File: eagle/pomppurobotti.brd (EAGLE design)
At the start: 100 x 80 mm, 3 parts

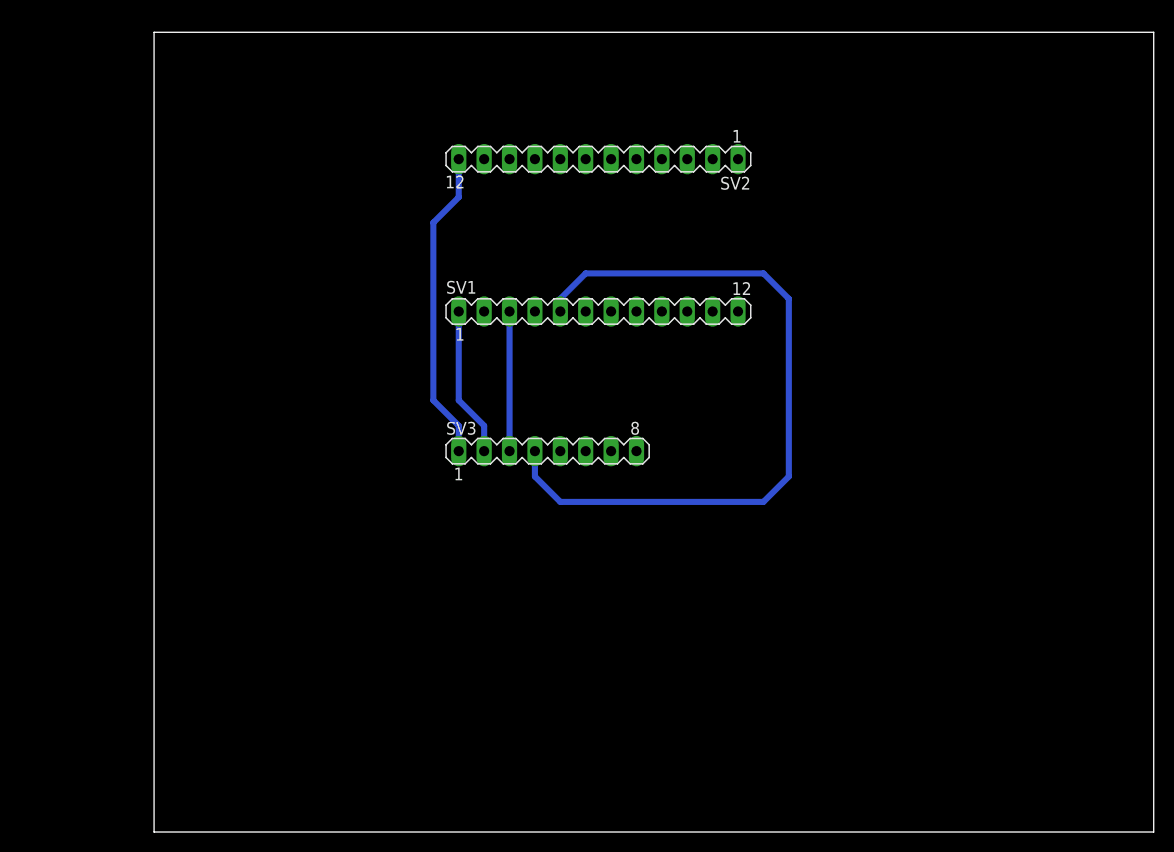
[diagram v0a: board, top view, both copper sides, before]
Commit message: First version of PCB
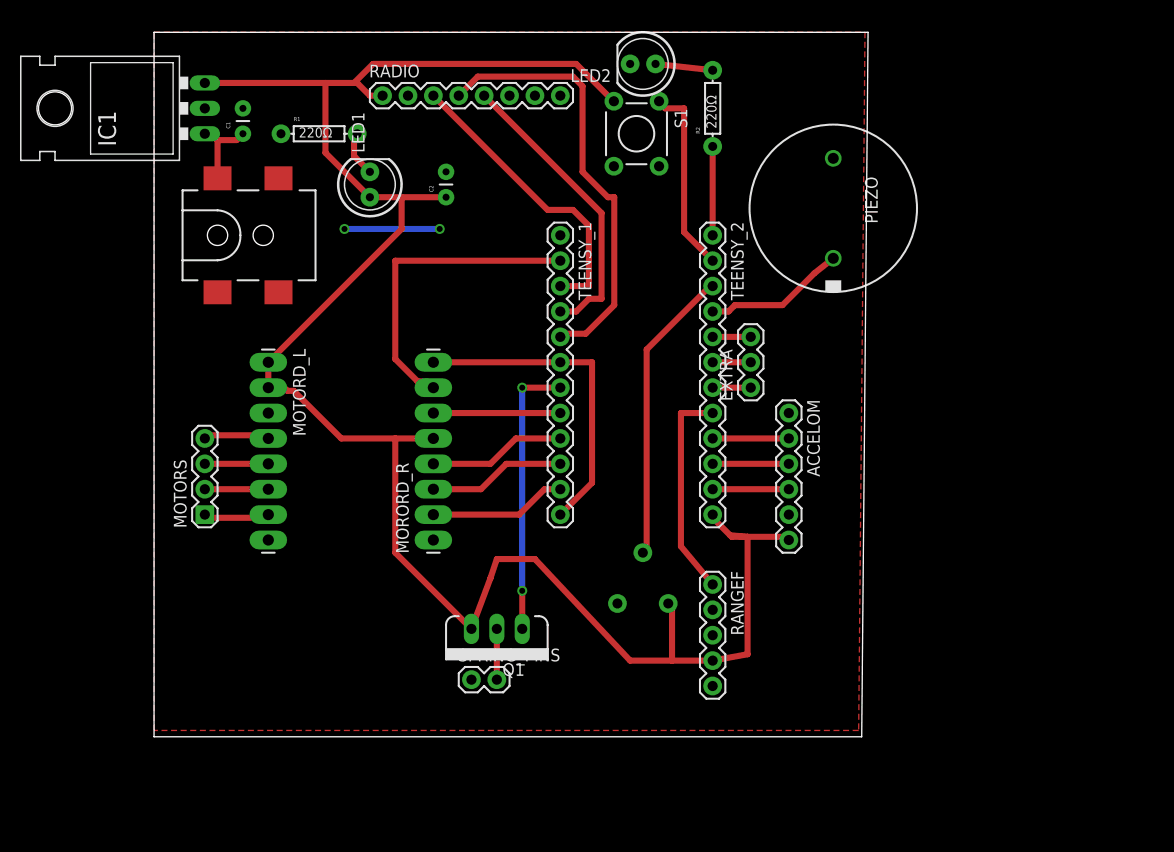
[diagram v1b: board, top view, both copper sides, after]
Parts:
- removed SV1, SV2: (no value), con-lstb:MA12-1
- removed SV3: (no value), con-lstb:MA08-1
- added ACCELOM: (no value), SparkFun-Connectors:1X06
- added C1, C2: 10uF, SparkFun-Capacitors:CAP-PTH-SMALL
- added EXTRA: (no value), SparkFun-Connectors:1X03
- added IC1: (no value), SparkFun-PowerIC:TO-220-ALT
- added JP1: POWER_JACK1, SparkFun-Connectors:POWER_JACK_SMD_OVERPASTE_REDBOARD_0603
- added LED1, LED2: RED, SparkFun-LED:LED5MM
- added MORORD_R, MOTORD_L: (no value), SparkFun-Connectors:1X08_LONGPADS
- added MOTORS: (no value), SparkFun-Connectors:1X04
- added PIEZO: EFBAA40D101, buzzer:EFBAA40D101
- added Q1: MOSFET-NCHANNELFQP30N06L, SparkFun-DiscreteSemi:TO220V
- added R1, R2: 220Ω, SparkFun-Resistors:AXIAL-0.3
- added RADIO: (no value), SparkFun-Connectors:1X08_ROUND
- added RANGEF: (no value), SparkFun-Connectors:1X05
- added RV1: (no value), SparkFun-Electromechanical:TRIM_POT
- added S1: SWITCH-MOMENTARY-2PTH, SparkFun-Electromechanical:TACTILE-PTH
- added SPRING_PINS: M02PTH, SparkFun-Connectors:1X02
- added TEENSY_1, TEENSY_2: M12PTH, SparkFun-Connectors:1X12
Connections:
- removed net +5V: SV2.12, SV3.1
- removed net 0: SV1.2
- removed net 10: SV1.12
- removed net 4: SV1.6
- removed net 5: SV1.7
- removed net 6: SV1.8
- removed net 7: SV1.9
- removed net 8: SV1.10
- removed net 9: SV1.11
- removed net N$14: SV2.11
- removed net N$15: SV2.10
- removed net N$16: SV2.9
- removed net N$17: SV2.8
- removed net N$18: SV2.7
- removed net N$19: SV2.6
- removed net N$20: SV2.5
- removed net N$21: SV2.4
- removed net N$22: SV2.3
- removed net N$23: SV2.2
- removed net N$24: SV2.1
- new net A0: ACCELOM.2, TEENSY_2.9
- new net A01: MOTORD_L.4, MOTORS.4
- new net A02: MOTORD_L.5, MOTORS.3
- new net A1: ACCELOM.3, TEENSY_2.10
- new net A2: ACCELOM.4, TEENSY_2.11
- new net A4: EXTRA.1, TEENSY_2.7
- new net A5: EXTRA.2, TEENSY_2.6
- new net A8: RV1.1, TEENSY_2.3
- new net AIN1: MORORD_R.6, TEENSY_1.8
- new net AIN2: MORORD_R.7, TEENSY_1.2
- new net AN: RANGEF.1, TEENSY_2.8
- new net B01: MOTORD_L.7, MOTORS.1
- new net B02: MOTORD_L.6, MOTORS.2
- new net BIN1: MORORD_R.4, TEENSY_1.9
- new net BIN2: MORORD_R.3, TEENSY_1.10
- new net LEDA10: R2.P$1, TEENSY_2.1
- new net N$2: LED1.K, R1.P$2
- new net N$3: C1.1, IC1.IN, JP1.VIN0
- new net N$4: LED2.A, R2.P$2
- new net N$5: Q1.2, SPRING_PINS.2
- new net PWMA: MORORD_R.8, TEENSY_1.12, TEENSY_1.6
- new net PWMA6: EXTRA.3, TEENSY_2.5
- new net PWMA7: PIEZO.2, TEENSY_2.4
- new net PWMA9: S1.1, TEENSY_2.2
- new net PWMB: MORORD_R.2, TEENSY_1.11
- new net PWMC: Q1.1, TEENSY_1.7
- new net VCC: ACCELOM.6, C2.1, IC1.OUT, LED1.A, MORORD_R.5, MOTORD_L.1, MOTORD_L.2, Q1.3, RADIO.1, RANGEF.4, RV1.3, S1.3, TEENSY_2.12
- net +3.3V: now also RADIO.8; no longer SV3.8
- net GND: now also ACCELOM.5, C1.2, C2.2, IC1.GND, JP1.P$4, LED2.K, MORORD_R.1, MOTORD_L.3, MOTORD_L.8, PIEZO.1, R1.P$1, RADIO.2, RANGEF.5, RV1.2, SPRING_PINS.1, TEENSY_1.1; no longer SV1.1, SV3.2
- net IRQ: now also RADIO.7; no longer SV3.7
- net MISO: now also RADIO.4, TEENSY_1.5; no longer SV1.5, SV3.4
- net MOSI: now also RADIO.5, TEENSY_1.4; no longer SV1.4, SV3.5
- net SCLK: now also RADIO.3, TEENSY_1.3; no longer SV1.3, SV3.3
- net SEL: now also RADIO.6; no longer SV3.6
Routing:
- net VCC: track 0.00 -> 198.5 mm
- net PWMA: track 0.00 -> 32.4 mm
- net AIN2: track 0.00 -> 31.3 mm
- net +5V: track 31.3 -> 0.00 mm
- net A8: track 0.00 -> 30.3 mm
- net MISO: track 74.1 -> 43.9 mm
- net MOSI: track 0.00 -> 29.8 mm
- net PWMC: track 0.00 -> 27.9 mm, vias 0 -> 2
- net AN: track 0.00 -> 21.5 mm
- net PWMA9: track 0.00 -> 19.3 mm
- net SCLK: track 14.0 -> 29.8 mm
- net PWMA7: track 0.00 -> 14.2 mm
- net PWMB: track 0.00 -> 13.8 mm
- net BIN2: track 0.00 -> 13.8 mm
- net BIN1: track 0.00 -> 13.8 mm
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- added copper zone on layer 1, net GND
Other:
- board size 100 x 80 mm -> 71.4 x 70.5 mm

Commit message: Many major improvements
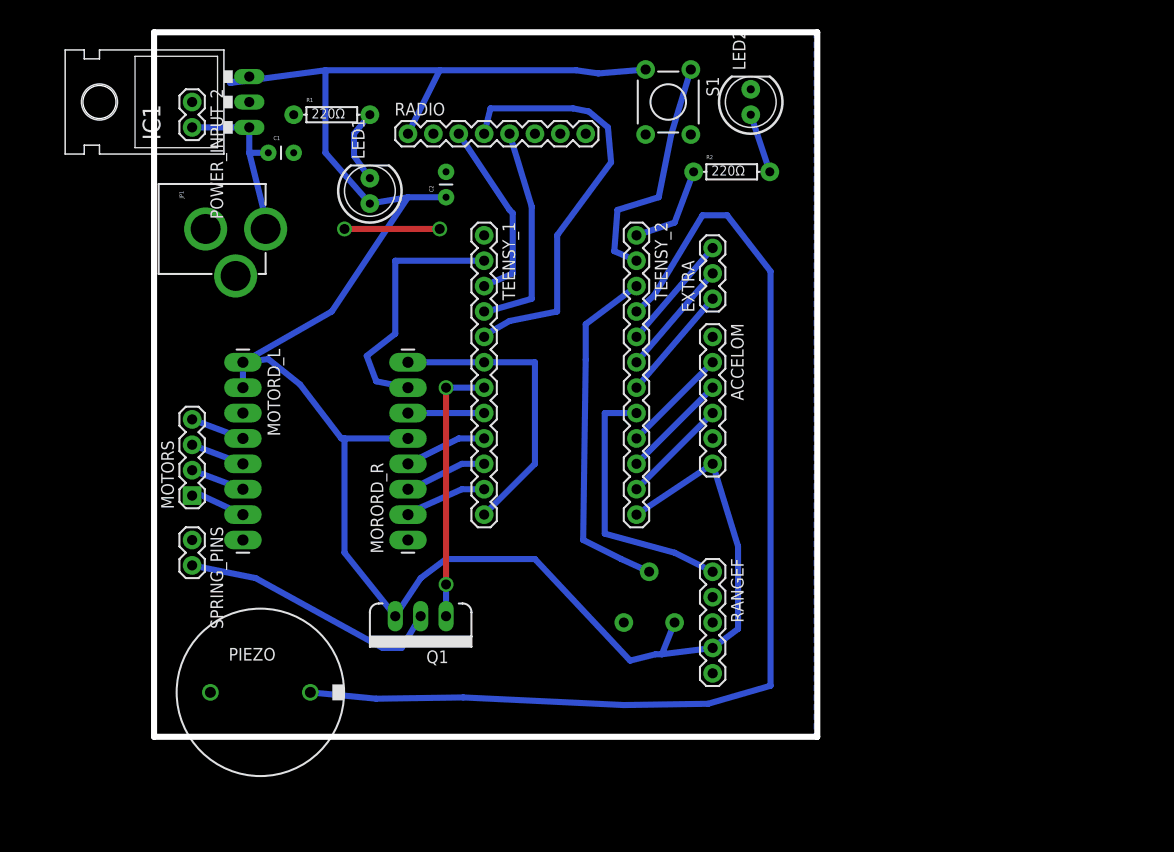
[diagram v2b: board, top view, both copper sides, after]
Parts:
- added POWER_INPUT_2: M02PTH, SparkFun-Connectors:1X02
- JP1: value POWER_JACK1 -> POWER_JACKPTH; device SparkFun-Connectors:POWER_JACK_SMD_OVERPASTE_REDBOARD_0603 -> SparkFun-Connectors:POWER_JACK_PTH
- moved PIEZO 75.0 mm to (10.6, 14.0), turned to 0 degrees
- moved SPRING_PINS 31.2 mm to (3.81, 29.2), turned to 270 degrees
- moved LED2 11.4 mm to (59.7, 73.0), turned to 90 degrees
- moved ACCELOM 10.8 mm to (55.9, 49.5)
- moved EXTRA 9.67 mm to (55.9, 53.3)
- moved JP1 8.91 mm to (-2.54, 60.3), turned to 270 degrees
- moved Q1 7.73 mm to (26.7, 21.6)
- moved TEENSY_2 7.62 mm to (48.3, 59.7)
- moved TEENSY_1 7.62 mm to (33.0, 59.7)
- moved R2 6.63 mm to (57.8, 66.0), turned to 0 degrees
- moved RADIO 4.58 mm to (25.4, 69.8)
- moved S1 4.49 mm to (51.4, 73.0)
- moved IC1 4.49 mm to (5.71, 73.0)
- moved C1 3.18 mm to (11.4, 67.9), turned to 0 degrees
- moved MORORD_R 2.54 mm to (25.4, 29.2)
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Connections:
- net GND: now also JP1.GND, POWER_INPUT_2.1; no longer JP1.P$4
- net N$3: now also JP1.PWR, POWER_INPUT_2.2; no longer JP1.VIN0
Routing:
- net PWMA7: track 14.2 -> 109.1 mm
- net N$5: track 5.08 -> 26.6 mm
- net VCC: track 198.5 -> 211.2 mm
- net SCLK: track 29.8 -> 18.8 mm
- net N$3: track 8.16 -> 18.0 mm
- net MOSI: track 29.8 -> 21.8 mm
- net PWMA6: track 3.81 -> 11.7 mm
- net A5: track 3.81 -> 11.7 mm
- net A4: track 3.81 -> 11.7 mm
- net AIN2: track 31.3 -> 25.8 mm
- net BIN2: track 13.8 -> 8.22 mm
- net BIN1: track 13.8 -> 8.22 mm
- net AN: track 21.5 -> 26.7 mm
- net AIN1: track 12.7 -> 7.62 mm
- net A8: track 30.3 -> 35.3 mm
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- added copper zone on layer 16, net GND
- removed copper zone on layer 1, net GND
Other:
- board size 71.4 x 70.5 mm -> 66.3 x 70.5 mm
